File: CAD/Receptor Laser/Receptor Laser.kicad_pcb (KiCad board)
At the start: 2 copper layers, 115 parts

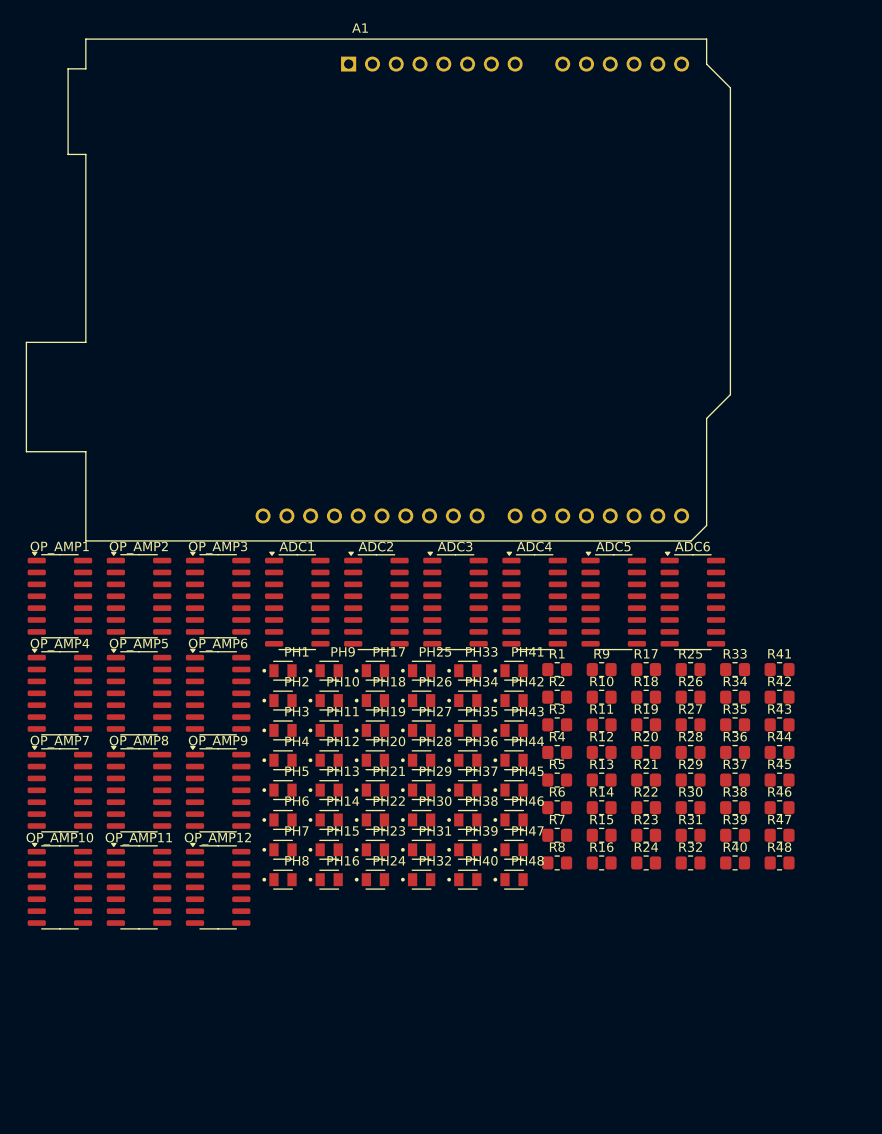
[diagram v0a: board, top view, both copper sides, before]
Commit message: a
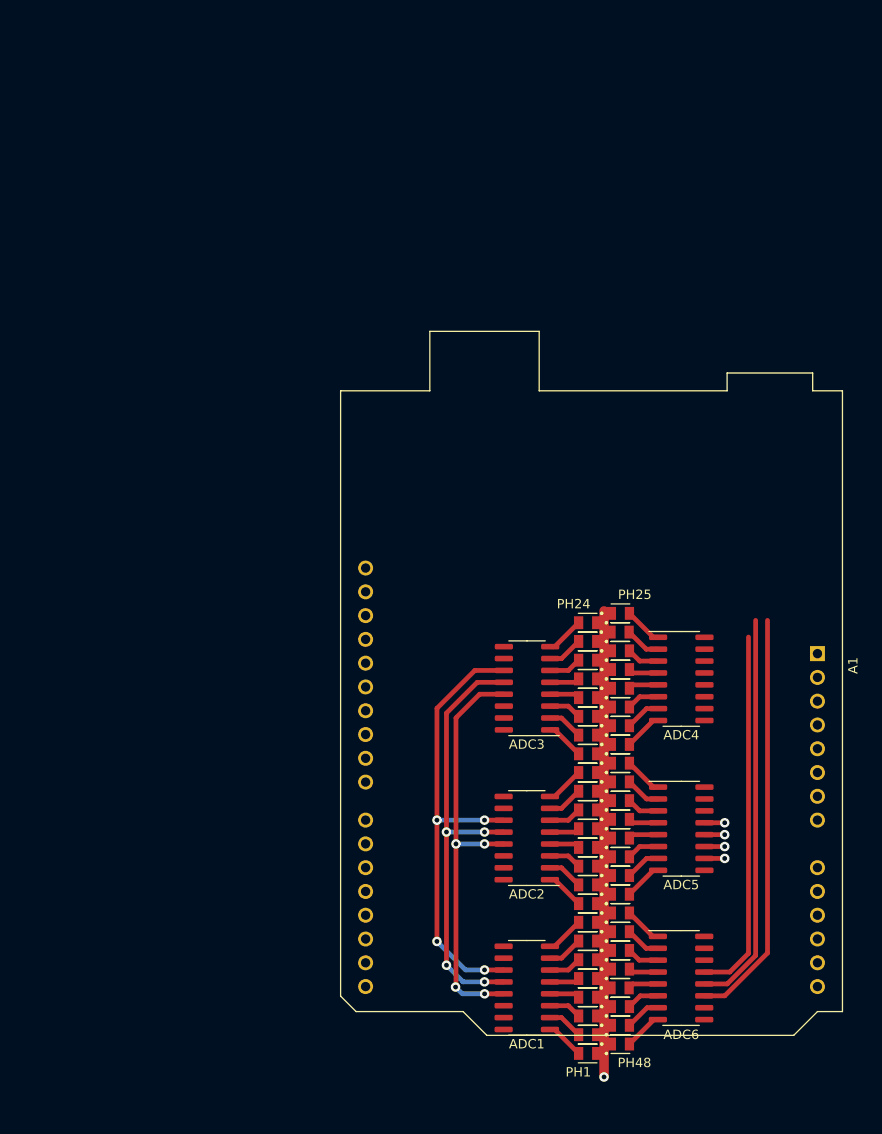
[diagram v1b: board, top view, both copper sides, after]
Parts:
- removed OP_AMP1, OP_AMP10, OP_AMP11, OP_AMP12, OP_AMP2, OP_AMP3, OP_AMP4, OP_AMP5, OP_AMP6, OP_AMP7, OP_AMP8, OP_AMP9: MC33079, Package_SO:SOIC-14_3.9x8.7mm_P1.27mm
- removed R1, R10, R11, R12, R13, R14, R15, R16, R17, R18, R19, R2, R20, R21, R22, R23, R24, R25, R26, R27, R28, R29, R3, R30, R31, R32, R33, R34, R35, R36, R37, R38, R39, R4, R40, R41, R42, R43, R44, R45, R46, R47, R48, R5, R6, R7, R8, R9: R, Resistor_SMD:R_0805_2012Metric_Pad1.20x1.40mm_HandSolder
- moved A1 80.4 mm to (98.0, 82.8), turned to -90 degrees
- moved PH1 52.2 mm to (73.5, 125.5), turned to 180 degrees
- moved PH2 48.3 mm to (73.5, 123.5), turned to 180 degrees
- moved ADC1 47.9 mm to (67.0, 118.5), turned to 180 degrees
- moved PH3 44.6 mm to (73.5, 121.5), turned to 180 degrees
- moved PH4 41.2 mm to (73.5, 119.5), turned to 180 degrees
- moved ADC6 40.2 mm to (83.5, 117.4)
- moved PH5 38.3 mm to (73.5, 117.5), turned to 180 degrees
- moved PH9 37.2 mm to (73.5, 109.5), turned to 180 degrees
- moved PH6 35.8 mm to (73.5, 115.5), turned to 180 degrees
- moved PH24 35.6 mm to (73.5, 79.5), turned to 180 degrees
- moved PH7 34.0 mm to (73.5, 113.5), turned to 180 degrees
- moved PH10 33.9 mm to (73.5, 107.5), turned to 180 degrees
- moved PH8 32.9 mm to (73.5, 111.5), turned to 180 degrees
- moved PH23 31.8 mm to (73.5, 81.5), turned to 180 degrees
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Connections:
- PH1 pad A: Net-(OP_AMP1A--) -> /PH-1
- PH10 pad A: Net-(OP_AMP3B--) -> /PH-10
- PH11 pad A: Net-(OP_AMP3C--) -> /PH-11
- PH12 pad A: Net-(OP_AMP3D--) -> /PH-12
- PH13 pad A: Net-(OP_AMP4A--) -> /PH-13
- PH14 pad A: Net-(OP_AMP4B--) -> /PH-14
- PH15 pad A: Net-(OP_AMP4C--) -> /PH-15
- PH16 pad A: Net-(OP_AMP4D--) -> /PH-16
- PH17 pad A: Net-(OP_AMP5A--) -> /PH-17
- PH18 pad A: Net-(OP_AMP5B--) -> /PH-18
- PH19 pad A: Net-(OP_AMP5C--) -> /PH-19
- PH2 pad A: Net-(OP_AMP1B--) -> /PH-2
- PH20 pad A: Net-(OP_AMP5D--) -> /PH-20
- PH21 pad A: Net-(OP_AMP6A--) -> /PH-21
- PH22 pad A: Net-(OP_AMP6B--) -> /PH-22
- PH23 pad A: Net-(OP_AMP6C--) -> /PH-23
- PH24 pad A: Net-(OP_AMP6D--) -> /PH-24
- PH25 pad A: Net-(OP_AMP7A--) -> /PH-25
- PH26 pad A: Net-(OP_AMP7B--) -> /PH-26
- PH27 pad A: Net-(OP_AMP7C--) -> /PH-27
- PH28 pad A: Net-(OP_AMP7D--) -> /PH-28
- PH29 pad A: Net-(OP_AMP8A--) -> /PH-29
- PH3 pad A: Net-(OP_AMP1C--) -> /PH-3
- PH30 pad A: Net-(OP_AMP8B--) -> /PH-30
- PH31 pad A: Net-(OP_AMP8C--) -> /PH-31
- PH32 pad A: Net-(OP_AMP8D--) -> /PH-32
- PH33 pad A: Net-(OP_AMP9A--) -> /PH-33
- PH34 pad A: Net-(OP_AMP9B--) -> /PH-34
- PH35 pad A: Net-(OP_AMP9C--) -> /PH-35
- PH36 pad A: Net-(OP_AMP9D--) -> /PH-36
- PH37 pad A: Net-(OP_AMP10A--) -> /PH-37
- PH38 pad A: Net-(OP_AMP10B--) -> /PH-38
- PH39 pad A: Net-(OP_AMP10C--) -> /PH-39
- PH4 pad A: Net-(OP_AMP1D--) -> /PH-4
- PH40 pad A: Net-(OP_AMP10D--) -> /PH-40
- PH41 pad A: Net-(OP_AMP11A--) -> /PH-41
- PH42 pad A: Net-(OP_AMP11B--) -> /PH-42
- PH43 pad A: Net-(OP_AMP11C--) -> /PH-43
- PH44 pad A: Net-(OP_AMP11D--) -> /PH-44
- PH45 pad A: Net-(OP_AMP12A--) -> /PH-45
- PH46 pad A: Net-(OP_AMP12B--) -> /PH-46
- PH47 pad A: Net-(OP_AMP12C--) -> /PH-47
- PH48 pad A: Net-(OP_AMP12D--) -> /PH-48
- PH5 pad A: Net-(OP_AMP2A--) -> /PH-5
- PH6 pad A: Net-(OP_AMP2B--) -> /PH-6
- PH7 pad A: Net-(OP_AMP2C--) -> /PH-7
- PH8 pad A: Net-(OP_AMP2D--) -> /PH-8
- PH9 pad A: Net-(OP_AMP3A--) -> /PH-9
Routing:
- net /MOSI: track 0.00 -> 95.6 mm, vias 0 -> 5
- net /MISO: track 0.00 -> 92.1 mm, vias 0 -> 5
- net /CLK: track 0.00 -> 87.0 mm, vias 0 -> 5
- net +5V: track 0.00 -> 49.8 mm, vias 0 -> 1
- net /PH-9: track 0.00 -> 4.12 mm
- net /PH-8: track 0.00 -> 4.12 mm
- net /PH-40: track 0.00 -> 4.12 mm
- net /PH-33: track 0.00 -> 4.12 mm
- net /PH-32: track 0.00 -> 4.12 mm
- net /PH-25: track 0.00 -> 4.12 mm
- net /PH-16: track 0.00 -> 4.12 mm
- net /PH-1: track 0.00 -> 4.12 mm
- net /PH-48: track 0.00 -> 4.12 mm
- net /PH-24: track 0.00 -> 4.09 mm
- net /PH-17: track 0.00 -> 4.09 mm
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
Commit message: pcb receptor
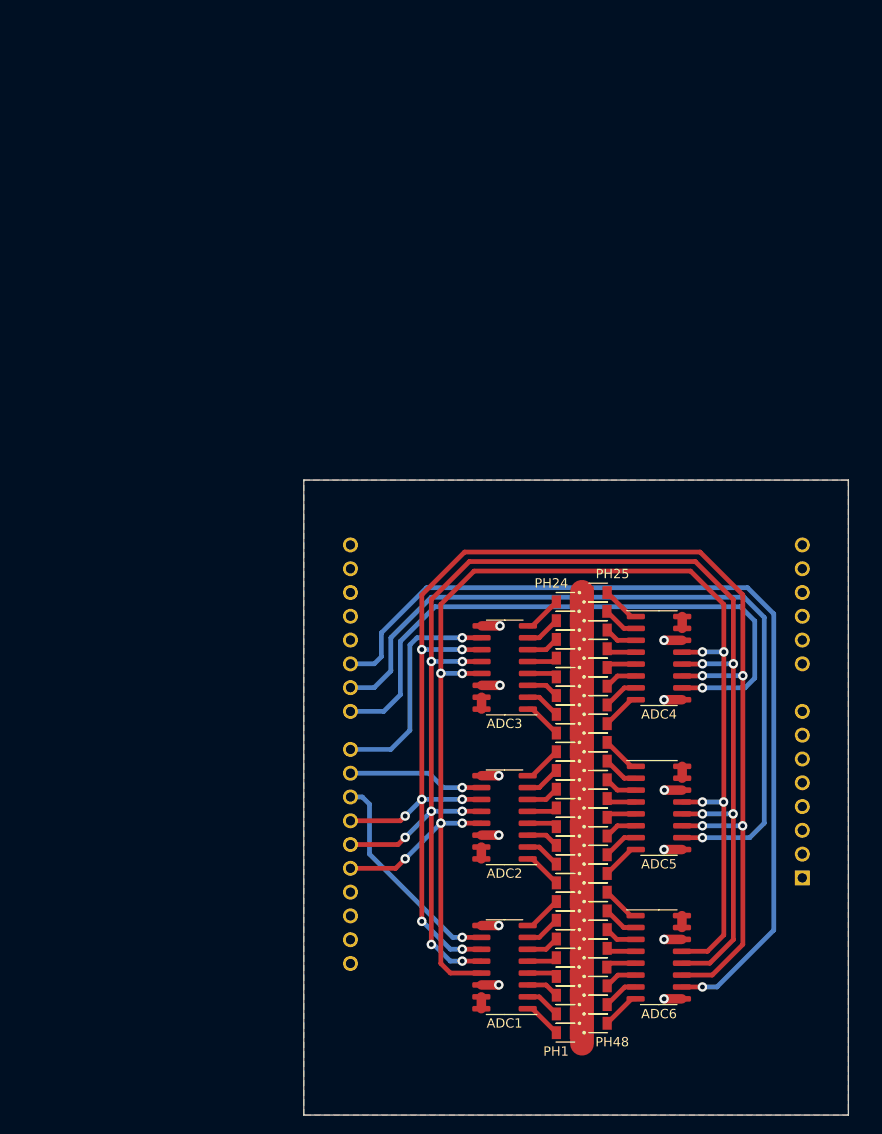
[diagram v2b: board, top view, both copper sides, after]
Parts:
- UNO1: renamed from A1; moved to B.Cu
- moved UNO1 24.0 mm to (96.4, 106.8), turned to 90 degrees
- moved ADC3 3.25 mm to (64.6, 84.3)
- moved PH26 3.25 mm to (74.6, 78.3)
- moved PH45 3.25 mm to (74.6, 116.3)
- moved ADC1 3.25 mm to (64.6, 116.3)
- moved ADC2 3.25 mm to (64.6, 100.3)
- moved ADC4 3.25 mm to (81.1, 83.3)
- moved ADC5 3.25 mm to (81.1, 99.3)
- moved PH1 3.25 mm to (71.1, 123.3)
- moved PH10 3.25 mm to (71.1, 105.3)
- moved PH11 3.25 mm to (71.1, 103.3)
- moved PH12 3.25 mm to (71.1, 101.3)
- moved PH13 3.25 mm to (71.1, 99.3)
- moved PH14 3.25 mm to (71.1, 97.3)
- moved PH15 3.25 mm to (71.1, 95.3)
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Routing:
- net /CS6: track 0.00 -> 97.3 mm, vias 0 -> 1
- net /CS5: track 2.16 -> 82.6 mm
- net /CS4: track 0.00 -> 66.1 mm, vias 0 -> 1
- net /MOSI: track 95.6 -> 160.0 mm, vias 5 -> 11
- net /MISO: track 92.1 -> 153.2 mm, vias 5 -> 11
- net /CLK: track 87.0 -> 146.0 mm, vias 5 -> 9
- net /CS3: track 0.00 -> 24.3 mm, vias 0 -> 1
- net /CS1: track 0.00 -> 23.3 mm, vias 0 -> 1
- net GND: track 0.00 -> 22.9 mm, vias 0 -> 12
- net /CS2: track 0.00 -> 14.6 mm, vias 0 -> 1
- net +5V: track 49.8 -> 55.9 mm, vias 1 -> 0
- added copper zone on F.Cu, net +5V
- added copper zone on B.Cu, net GND
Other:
- board outline added: 58.2 x 67.8 mm
